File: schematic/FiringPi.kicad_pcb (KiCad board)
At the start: 4 copper layers, 65 x 85.9 mm, 74 parts, among them IC1 HX711, J12 UART, P1 Raspberry Pi GPIO Header, Q1 MMBT4403, U4 LM2596S-5, U5 ADS1115IDGS, U6 MAX31865xAP, U7 MAX31865xAP

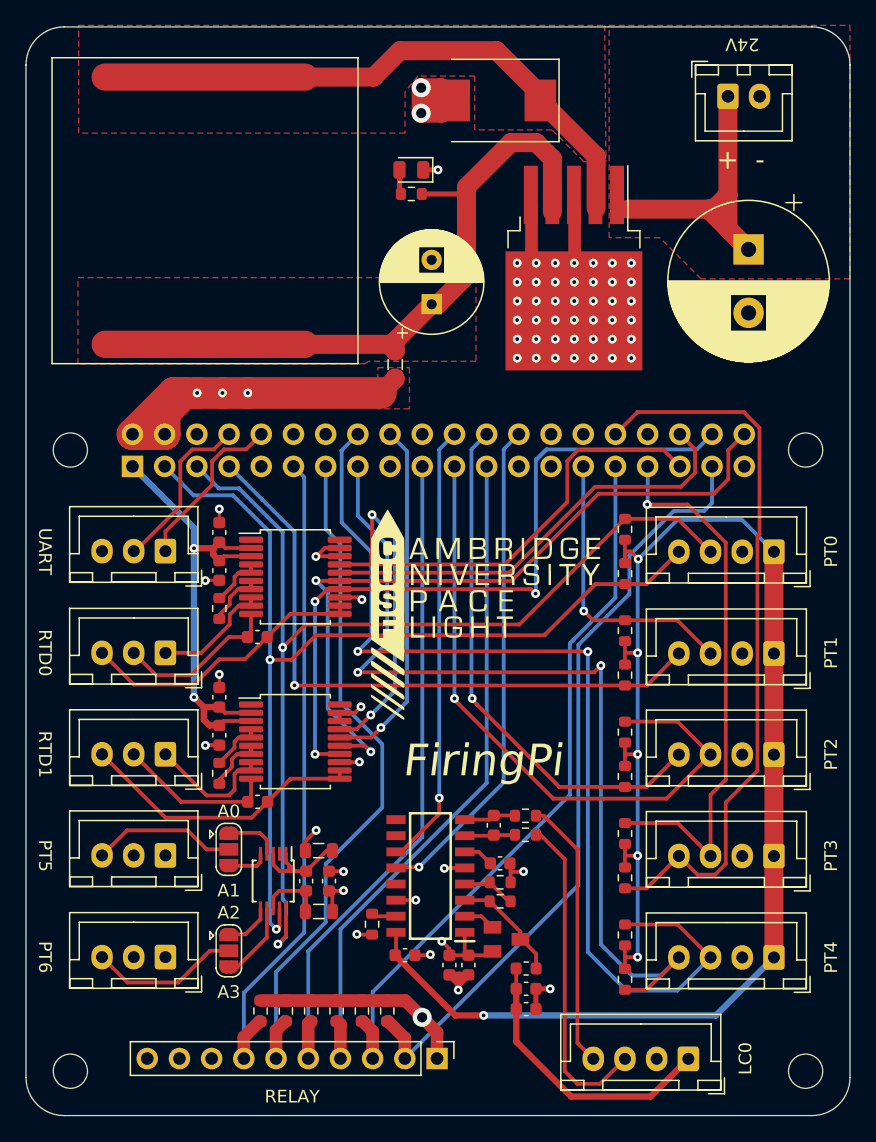
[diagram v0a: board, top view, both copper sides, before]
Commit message: Generated gerbers
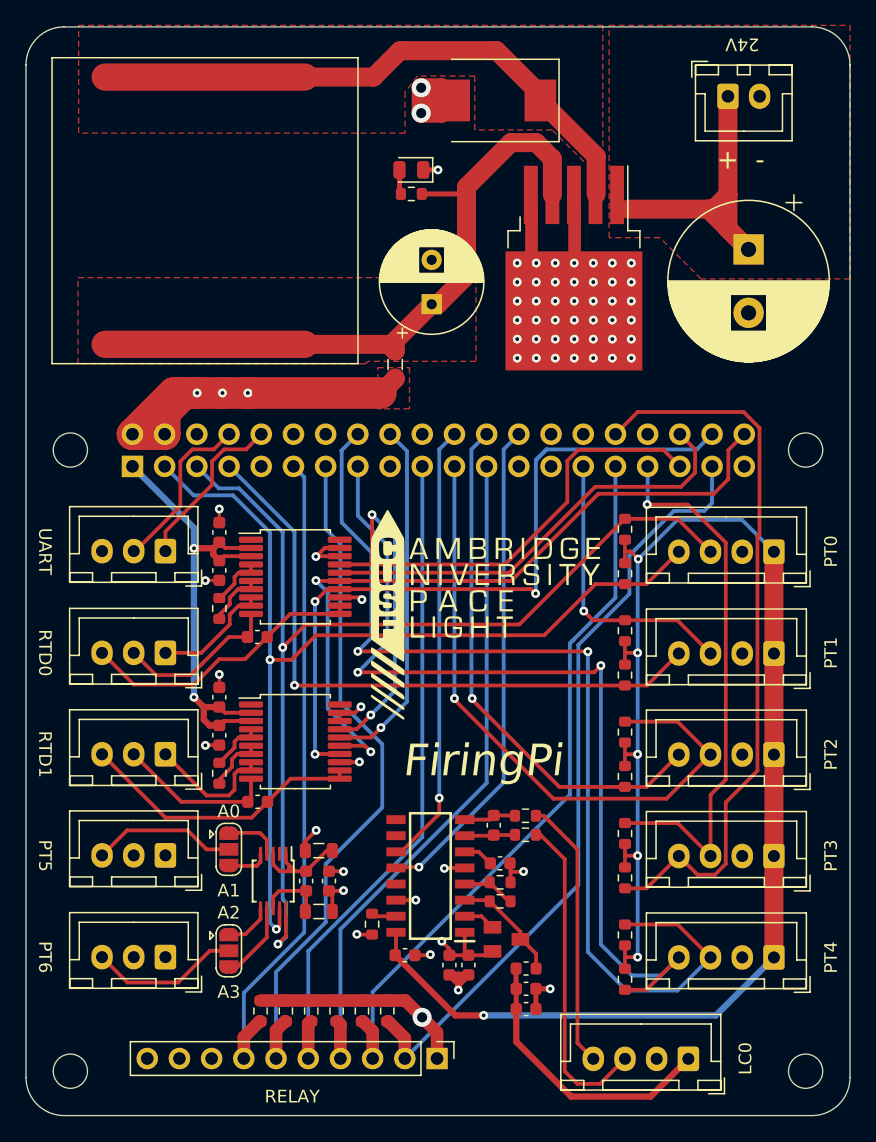
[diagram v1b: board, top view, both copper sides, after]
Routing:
- net Net-(C2-Pad1): track 47.5 -> 46.1 mm
- net Net-(D1-Pad1): track 39.5 -> 38.4 mm
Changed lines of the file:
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@@
   (via (at 39.75 60.65) (size 0.7) (drill 0.3) (layers "F.Cu" "B.Cu") (net 2))
   (segment (start 63.175 102.675) (end 63.175 100.1) (width 0.5) (layer "F.Cu") (net 3))
-  (segment (start 63.1625 96.9) (end 63.1625 98.7625) (width 0.3) (layer "F.Cu") (net 3))
-  (segment (start 63.175 100.1) (end 63.175 98.5) (width 0.5) (layer "F.Cu") (net 3))
+  (segment (start 63.175 98.5) (end 63.175 100.1) (width 0.4) (layer "F.Cu") (net 3))
   (segment (start 67.5 107) (end 73.775 107) (width 0.5) (layer "F.Cu") (net 3))
-  (segment (start 63.1625 98.7625) (end 63.2 98.8) (width 0.3) (layer "F.Cu") (net 3))
+  (segment (start 63.1625 96.9) (end 63.1625 98.4875) (width 0.4) (layer "F.Cu") (net 3))
   (segment (start 63.175 102.675) (end 67.5 107) (width 0.5) (layer "F.Cu") (net 3))
   (segment (start 73.775 107) (end 76.75 104.025) (width 0.5) (layer "F.Cu") (net 3))
@@
   (segment (start 61.625 24.5) (end 54 24.5) (width 1.5) (layer "F.Cu") (net 13))
   (segment (start 69.475 32.825) (end 65.075 28.425) (width 1.5) (layer "F.Cu") (net 13))
+  (segment (start 69.475 32.825) (end 69.475 35.825) (width 1.5) (layer "F.Cu") (net 13))
   (segment (start 51.91968 26.58032) (end 38.62132 26.58032) (width 1.5) (layer "F.Cu") (net 13))
-  (segment (start 69.475 36.925) (end 69.475 32.825) (width 1.5) (layer "F.Cu") (net 13))
   (segment (start 54 24.5) (end 51.91968 26.58032) (width 1.5) (layer "F.Cu") (net 13))
   (segment (start 60.425 92.775) (end 61.3 93.65) (width 0.3) (layer "F.Cu") (net 14))
@@
   (segment (start 55.725 35.8) (end 58.7 35.8) (width 0.4) (layer "F.Cu") (net 73))
   (segment (start 64.75 31.75) (end 62.75 31.75) (width 1.5) (layer "F.Cu") (net 73))
-  (segment (start 66.025 35.875) (end 66.025 33.025) (width 1.5) (layer "F.Cu") (net 73))
   (segment (start 66.025 33.025) (end 64.75 31.75) (width 1.5) (layer "F.Cu") (net 73))
   (segment (start 59.25 42.25) (end 57 44.5) (width 1.5) (layer "F.Cu") (net 73))
+  (segment (start 66.025 33.025) (end 66.025 35.875) (width 1.5) (layer "F.Cu") (net 73))
   (segment (start 53.09614 47.66232) (end 53.62132 48.1875) (width 1.5) (layer "F.Cu") (net 73))
   (segment (start 58.7 35.8) (end 59.25 35.25) (width 0.4) (layer "F.Cu") (net 73))
   (segment (start 57 44.5) (end 56.5 44.5) (width 1.5) (layer "F.Cu") (net 73))
-  (segment (start 66.025 35.875) (end 66.025 37.225) (width 1.5) (layer "F.Cu") (net 73))
   (segment (start 53.62132 47.37868) (end 56.5 44.5) (width 1.5) (layer "F.Cu") (net 73))
   (segment (start 53.62132 48.1875) (end 53.62132 47.37868) (width 1.5) (layer "F.Cu") (net 73))
@@
     (polygon
       (pts
-        (xy 70.25 33.25)
+        (xy 70 33.25)
         (xy 68.5 33.25)
         (xy 66 30.75)
@@
         (xy 28.65 31)
         (xy 28.65 22.5)
-        (xy 70.15 22.5)
+        (xy 70 22.5)
       )
     )
